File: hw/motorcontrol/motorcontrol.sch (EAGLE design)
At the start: 87 parts, among them U1 BTN8982TA, U10 BSS138BKS, U2 BTN8982TA, U3 BTN8982TA, U7 PTR08060W

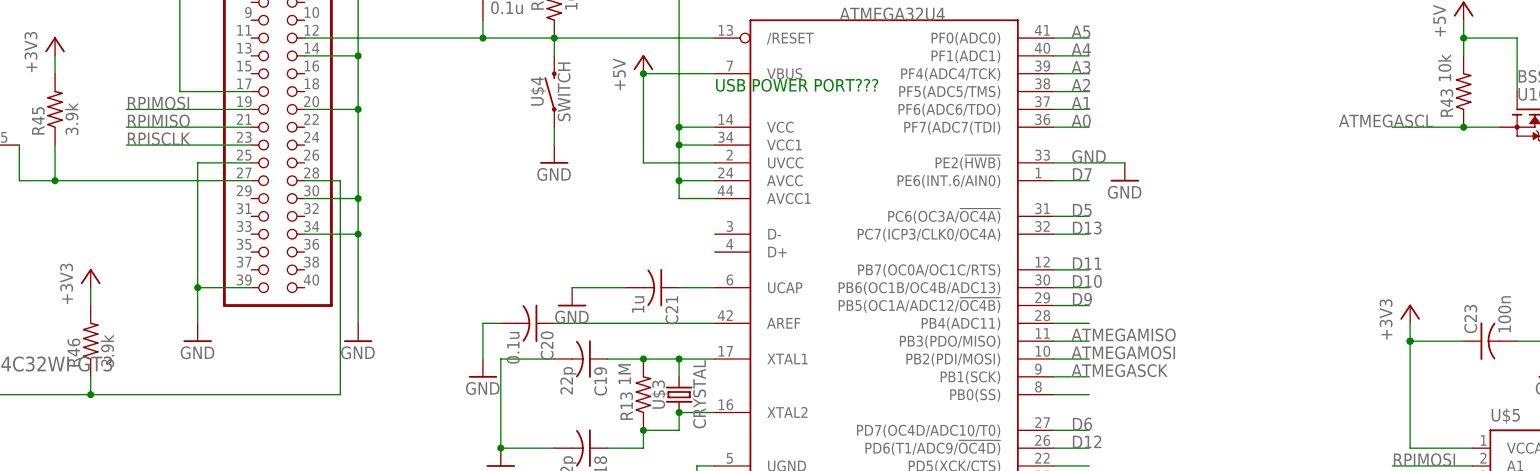
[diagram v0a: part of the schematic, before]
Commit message: schematics
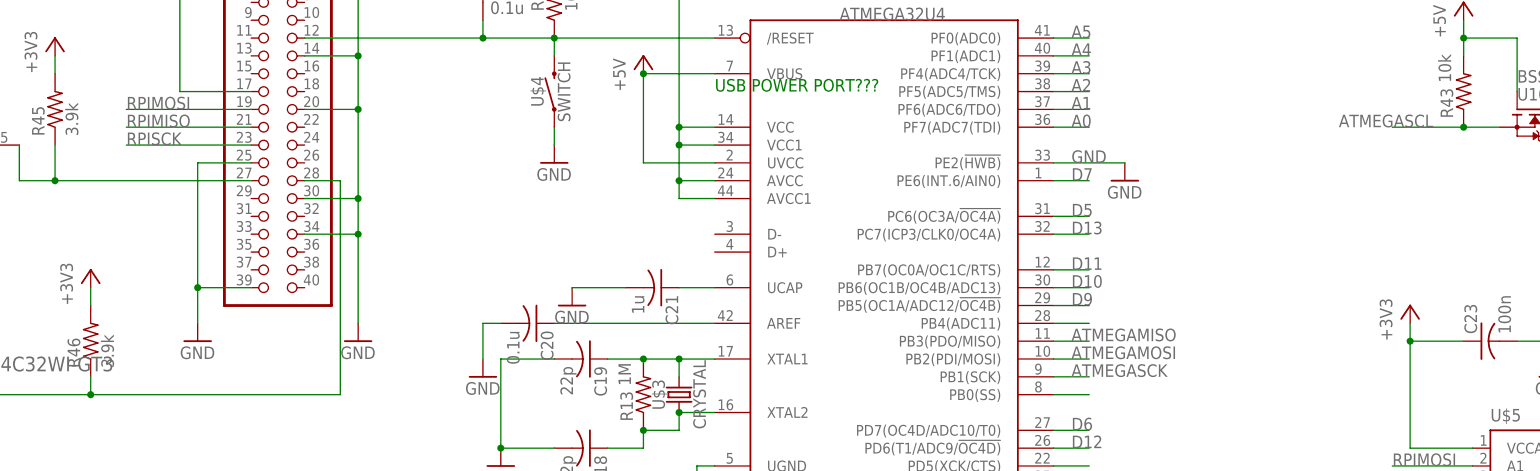
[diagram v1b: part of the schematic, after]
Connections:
- removed net RPISCLK: J2.23
- net RPISCK: now also J2.23
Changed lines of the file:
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@@
-</segment>
-</net>
-<net name="RPISCLK" class="0">
-<segment>
-<wire x1="-35.56" y1="129.54" x2="-53.34" y2="129.54" width="0.1524" layer="91"/>
-<label x="-53.34" y="129.54" size="1.778" layer="95"/>
-<pinref part="J2" gate="A" pin="23"/>
 </segment>
 </net>
@@
 <label x="127" y="78.74" size="1.778" layer="95"/>
 </segment>
-</net>
-<net name="N$2" class="0">
-<segment>
-<junction x="129.54" y="101.6"/>
-</segment>
-</net>
+<segment>
+<wire x1="-35.56" y1="129.54" x2="-53.34" y2="129.54" width="0.1524" layer="91"/>
+<label x="-53.34" y="129.54" size="1.778" layer="95"/>
+<pinref part="J2" gate="A" pin="23"/>
+</segment>
+</net>

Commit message: backup
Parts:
- removed DMG2305: DMG2305UX, rpibout:DMG2305UX
- removed EEPROM: EEPROM_CAT24C32WI-GT3, rpibout:EEPROM_CAT24C32WI-GT3
- removed JUMPER: 02JUMPER, rpibout:02JUMPER
- removed MMDT5401: MMDT5401, rpibout:MMDT5401
- removed U$1: IPD90P03P4L_04, rpibout:IPD90P03P4L_04
- removed U$5: ADG3304, rpibout:ADG3304
- added J1: (no value), pinhead:PINHD-1X2
- added U11: DMG2305UX, rpibout:DMG2305UX
- added U4: CAT24C32WI-GT3, rpibout:CAT24C32WI-GT3
- added U5: ADG3304, rpibout:ADG3304
- added U6: MMDT5401, rpibout:MMDT5401
- added U8: IPD90P03P4L_04, rpibout:IPD90P03P4L_04
- R15: value 1k -> 10k
- renumbered U$2 to U9
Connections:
- net N$8 renamed RPIRESET
- removed net N$10: EEPROM.SDA, J2.27, R45.1
- removed net N$42: DMG2305.G, MMDT5401.C1, R38.2
- removed net N$43: MMDT5401.B1, MMDT5401.B2, MMDT5401.C2, R37.2
- removed net N$7: EEPROM.SCL, J2.28, R46.1
- removed net VS: C11.1, C12.1, C13.1, C15.1, C16.+, C3.1, C7.1, D1.C, D2.C, U$1.S, U1.VS, U2.VS, U3.VS
- new net N$13: R37.2, U6G$1.B, U6G$1.C, U6G$2.B
- new net N$2: R38.2, U11.G, U6G$2.C
- new net RPISCL: J2.28, R46.1, U4.SCL
- new net RPISDA: J2.27, R45.1, U4.SDA
- new net VPP: C11.1, C12.1, C13.1, C15.1, C16.+, C3.1, C7.1, D1.C, D2.C, U1.VS, U2.VS, U3.VS, U8.S
- net +3V3: now also U4.VCC, U5.VCCA; no longer EEPROM.VCC, U$5.VCCA
- net +5V: now also U11.S, U5.EN, U5.VCCY, U6G$2.E; no longer DMG2305.S, MMDT5401.E1, U$5.EN, U$5.VCCY
- net ATMEGAMISO: now also U5.Y2; no longer U$5.Y2
- net ATMEGAMOSI: now also U5.Y1; no longer U$5.Y1
- net ATMEGASCK: now also U5.Y3; no longer U$5.Y3
- net GND: now also J1.2, U4.A0, U4.A1, U4.A2, U4.VSS, U5.GND; no longer EEPROM.A0, EEPROM.A1, EEPROM.A2, EEPROM.VSS, JUMPER.P1, U$5.GND
- net N$12: now also J1.1, U4.WP; no longer EEPROM.WP, JUMPER.P2
- net N$21: now also U8.G; no longer U$1.G
- net RPIMISO: now also U5.A2; no longer U$5.A2
- net RPIMOSI: now also U5.A1; no longer U$5.A1
- net RPISCK: now also U5.A3; no longer U$5.A3
- net VBATT: now also U8.D; no longer U$1.D
- net VOUT: now also U11.D, U6G$1.E; no longer DMG2305.D, MMDT5401.E2
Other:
- note added: "5V Voltage Regulator and Backpower Protection"
- note added: "Motor Backpower Protection"
- note added: "Motor Controller"
- note added: "Raspberry Pi Hat EEPROM"
- note removed: "5V power indicator"
- note removed: "ARDUINO/RPI POWER SOURCE"
- note removed: "MOTOR_CONTROLLER POWER SOURCE"
- note removed: "MOTOR_CONTROLLER_1"
- moved on the sheet: BATT1, C1, C10, C11, C12, C13, C14, C15, C16, C17, C18, C19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

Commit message: motorcontrol schematic should be ready
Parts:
- removed ENC1: 22-23-2041, con-molex:22-23-2041
- removed MOTOR_CONN1, SERVO_MOTOR: ULTRAFIT_3CIRC, rpibout:ULTRAFIT_3CIRC
- removed U$3: CRYSTAL, rpibout:CRYSTAL
- removed U$4: SWITCH, rpibout:SWITCH
- added C25, C26, C27, C28, C29: 1u, resistor:C-USC1206
- added ENCODER: 22-23-2041, con-molex:22-23-2041
- added J3: SWITCH, rpibout:SWITCH
- added J4: ULTRAFIT_3CIRC, rpibout:ULTRAFIT_3CIRC
- added SERVO: 22-23-2031, con-molex:22-23-2031
- added U12: CRYSTAL, rpibout:CRYSTAL
- C23, C24: value 100n -> 0.1u
- R26, R27: value (none) -> 3.9k
- R30, R31, R43, R44: value 10k -> 3.9k
- U8: value IPD90P03P4L_04 -> IPD90P03P4L-04; device rpibout:IPD90P03P4L_04 -> rpibout:IPD90P03P4L-04
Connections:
- net RPISCL renamed RPIROMSCL
- net RPISDA renamed RPIROMSDA
- new net ATMEGARESET: C22.2, J3.2, R48.1, U5.Y4, U9./RESET
- net +3V3: now also J2.1
- net +5V: now also C25.1, C26.1, C27.1, C28.1, C29.1, ENCODER-1.S, SERVO-1.S, U6T2.E; no longer ENC1-1.S, SERVO_MOTOR.P1, U6G$2.E
- net D13: now also SERVO-2.S; no longer SERVO_MOTOR.P2
- net D4: now also ENCODER-3.S; no longer ENC1-3.S
- net D5: now also ENCODER-4.S; no longer ENC1-4.S
- net GND: now also C25.2, C26.2, C27.2, C28.2, C29.2, ENCODER-2.S, J2.9, J3.1, SERVO-3.S; no longer ENC1-2.S, SERVO_MOTOR.P3, U$4.1
- net N$13: now also U6T1.B, U6T1.C, U6T2.B; no longer U6G$1.B, U6G$1.C, U6G$2.B
- net N$16: now also U12.1; no longer U$3.1
- net N$2: now also U6T2.C; no longer U6G$2.C
- net N$3: now also U12.2; no longer U$3.2
- net OUT1: now also J4.P1; no longer MOTOR_CONN1.P1
- net OUT2: now also J4.P2; no longer MOTOR_CONN1.P2
- net OUT3: now also J4.P3; no longer MOTOR_CONN1.P3
- net RPIRESET: now also U5.A4; no longer C22.2, R48.1, U$4.2, U9./RESET
- net VOUT: now also U6T1.E; no longer U6G$1.E
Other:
- note removed: "5V Voltage Regulator and Backpower Protection"
- note removed: "Motor Controller"
- note removed: "Raspberry Pi GPIO"
- note removed: "Raspberry Pi Hat EEPROM"
- moved on the sheet: BATT1, C1, C10, C11, C12, C13, C14, C15, C16, C17, C18, C19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
